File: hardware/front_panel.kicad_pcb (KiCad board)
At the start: 2 copper layers, 9.8 x 128.5 mm, 4 parts

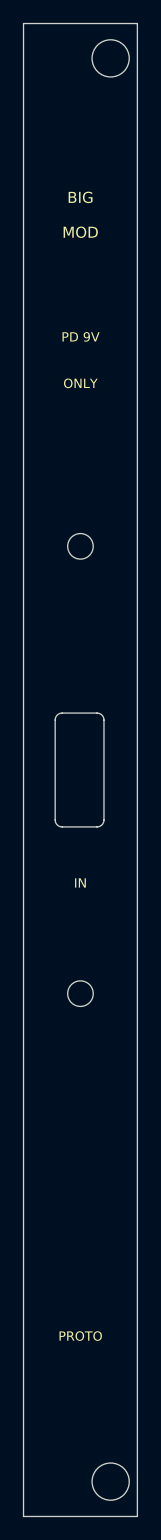
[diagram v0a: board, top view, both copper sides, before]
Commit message: Update on the PCB.
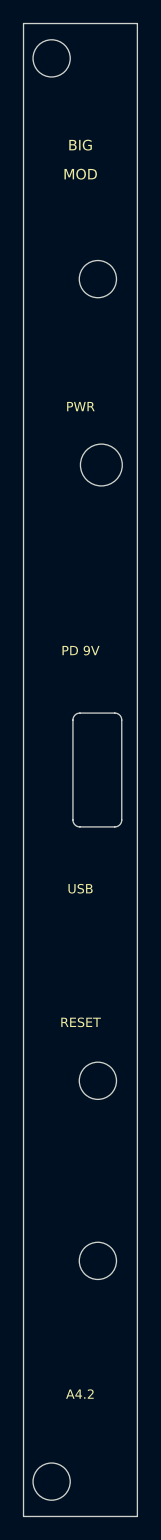
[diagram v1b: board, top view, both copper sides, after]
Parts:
- added H5: MECHANICAL_NPTH, , F.Cu at (56.7, 68.0)
- added H6: MECHANICAL_NPTH, , F.Cu at (56.4, 121.0)
- moved H3 23.0 mm to (56.4, 52.0)
- moved H4 23.0 mm to (56.4, 136.5)
- moved H1 5.08 mm to (52.4, 33.0)
- moved H2 5.08 mm to (52.4, 155.5)
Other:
- outline, holes or cut-outs redrawn
- board text added: "2HP / round corner holes X2.42 = X7.50 minus one 5.08mm rail pitch"
- board text added: "A4.2"
- board text added: "A4.2 plain L brackets: M3x8 panel / M3x8 countersunk side"
- board text added: "PWR"
- board text added: "RESET"
- board text added: "TL3340AF160QG SMT recessed reset; 3mm THT LED formed 90 degrees"
- board text added: "USB"
- board text removed: "2HP: 9.8 x 128.5 x 1.6 mm"
- board text removed: "Doepfer X=7.5 / dia3.2: 0.7mm FR4 web; M3 head overhang BLOCKER"
- board text removed: "Front face Z=0; inward +Z; NO copper"
- board text removed: "IN"
- board text removed: "Mounting proposal: ../docs/assembly.svg / mechanics.md"
- board text removed: "ONLY"
- board text removed: "PROTO"
- board text removed: "Port axis (X,Y,Z)=(4.900,64.250,0.800)"
- board text removed: "USB cutout: 4.2 x 9.8, R0.6"
